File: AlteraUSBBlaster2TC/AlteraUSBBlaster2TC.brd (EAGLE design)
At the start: 39.4 x 34 mm, 13 parts, among them U1 NCP1117LPST33T3G

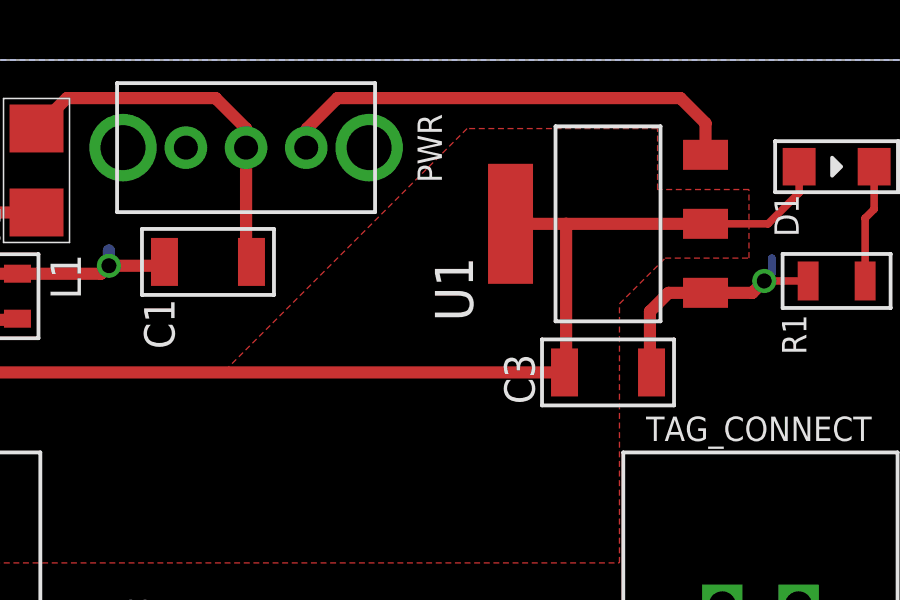
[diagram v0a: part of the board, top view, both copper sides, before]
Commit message: Major revamp of repo.
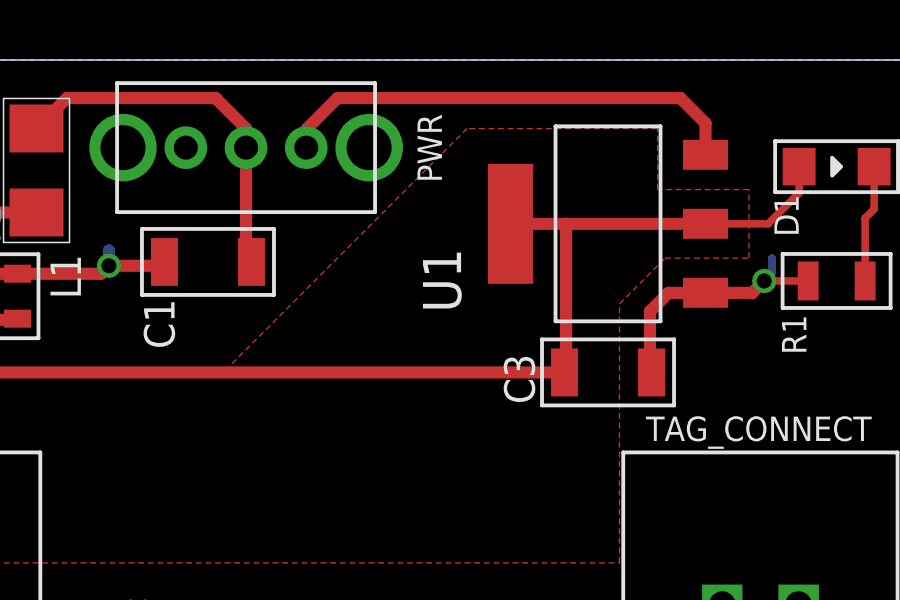
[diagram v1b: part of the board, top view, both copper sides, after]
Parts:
- turned U1 to 180 degrees
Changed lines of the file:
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@@
 <?xml version="1.0" encoding="utf-8"?>
 <!DOCTYPE eagle SYSTEM "eagle.dtd">
-<eagle version="7.6.0">
+<eagle version="7.4.0">
 <drawing>
 <settings>
@@
 <attribute name="MPN" value="5103308-1" x="33.655" y="10.795" size="1.778" layer="27" rot="R270" display="off"/>
 <attribute name="POPULATE" value="1" x="33.655" y="10.795" size="1.778" layer="27" rot="R270" display="off"/>
+<attribute name="VALUE" value="5103308-1" x="33.655" y="10.795" size="1.778" layer="27" rot="R270" display="off"/>
+<attribute name="HOUSEPART" value="" x="33.655" y="10.795" size="1.778" layer="27" rot="R270" display="off"/>
+<attribute name="URL" value="" x="33.655" y="10.795" size="1.778" layer="27" rot="R270" display="off"/>
 </element>
 <element name="USB_BLASTER" library="PP_Connectors" package="5103308-1" value="5103308-1" x="5.08" y="10.795" smashed="yes" rot="R270">
@@
 <attribute name="MPN" value="5103308-1" x="5.08" y="10.795" size="1.778" layer="27" rot="R270" display="off"/>
 <attribute name="POPULATE" value="1" x="5.08" y="10.795" size="1.778" layer="27" rot="R270" display="off"/>
+<attribute name="VALUE" value="5103308-1" x="5.08" y="10.795" size="1.778" layer="27" rot="R270" display="off"/>
+<attribute name="HOUSEPART" value="" x="5.08" y="10.795" size="1.778" layer="27" rot="R270" display="off"/>
+<attribute name="URL" value="" x="5.08" y="10.795" size="1.778" layer="27" rot="R270" display="off"/>
 </element>
 <element name="USB" library="MF_Connectors" package="MICROUSB-RIGHT" value="MF-CON-MICROUSB-RIGHT" x="2.921" y="28.575" rot="R270">
@@
 <attribute name="VALUE" value="MF-CON-MICROUSB-RIGHT" x="2.921" y="28.575" size="1.778" layer="27" rot="R270" display="off"/>
 </element>
-<element name="U1" library="MF_IC_Power" package="SOT-223-3" value="NCP1117LPST33T3G" x="28.575" y="28.575" smashed="yes" rot="R90">
-<attribute name="NAME" x="24.075" y="25.325" size="1.27" layer="25" font="vector" ratio="16" rot="R90"/>
-<attribute name="MPN" value="NCP1117LPST33T3G" x="28.575" y="28.575" size="1.778" layer="27" rot="R90" display="off"/>
-<attribute name="HOUSEPART" value="NO" x="28.575" y="28.575" size="1.778" layer="27" rot="R90" display="off"/>
-<attribute name="POPULATE" value="1" x="28.575" y="28.575" size="1.778" layer="27" rot="R90" display="off"/>
-<attribute name="URL" value="http://www.onsemi.com/pub_link/Collateral/NCP1117LP-D.PDF" x="28.575" y="28.575" size="1.778" layer="27" rot="R90" display="off"/>
-<attribute name="VALUE" value="NCP1117LPST33T3G" x="28.575" y="28.575" size="1.778" layer="27" rot="R90" display="off"/>
+<element name="U1" library="MF_IC_Power" package="SOT-223-3" value="NCP1117LPST33T3G" x="28.575" y="28.575" smashed="yes" rot="R180">
+<attribute name="NAME" x="22.407" y="27.761" size="1.27" layer="25" font="vector" ratio="16" rot="R270"/>
+<attribute name="MPN" value="NCP1117LPST33T3G" x="28.575" y="28.575" size="1.778" layer="27" rot="R180" display="off"/>
+<attribute name="HOUSEPART" value="NO" x="28.575" y="28.575" size="1.778" layer="27" rot="R180" display="off"/>
+<attribute name="POPULATE" value="1" x="28.575" y="28.575" size="1.778" layer="27" rot="R180" display="off"/>
+<attribute name="URL" value="http://www.onsemi.com/pub_link/Collateral/NCP1117LP-D.PDF" x="28.575" y="28.575" size="1.778" layer="27" rot="R180" display="off"/>
+<attribute name="VALUE" value="NCP1117LPST33T3G" x="28.575" y="28.575" size="1.778" layer="27" rot="R180" display="off"/>
 </element>
 <element name="F1" library="PP_Passives" package="1206" value="0ZCJ0010FF2E" x="9.525" y="30.353" rot="R90">
@@
 <attribute name="VALUE" value="" x="36.195" y="26.67" size="1.778" layer="27" rot="R180" display="off"/>
 </element>
-<element name="U$3" library="PP_Aesthetics" package="MF_LOGO_MEDIUM" value="MF_LOGOLOGO_MEDIUM" x="28.194" y="7.112" rot="R90"/>
+<element name="U$3" library="PP_Aesthetics" package="MF_LOGO_MEDIUM" value="MF_LOGOLOGO_MEDIUM" x="28.194" y="7.112" rot="R90">
+<attribute name="POPULATE" value="0" x="28.194" y="7.112" size="1.778" layer="27" rot="R90" display="off"/>
+<attribute name="MPN" value="" x="28.194" y="7.112" size="1.778" layer="27" rot="R90" display="off"/>
+</element>
 <element name="C1" library="MF_Passives" package="C1206" value="10uF" x="15.24" y="27.305" smashed="yes" rot="R180">
 <attribute name="TOLERANCE" value="" x="15.24" y="27.305" size="1.778" layer="27" rot="R180" display="off"/>
